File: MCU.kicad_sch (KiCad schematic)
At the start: 12 parts, among them IC2 PIC16F15345-I/SO, J5 490107670612

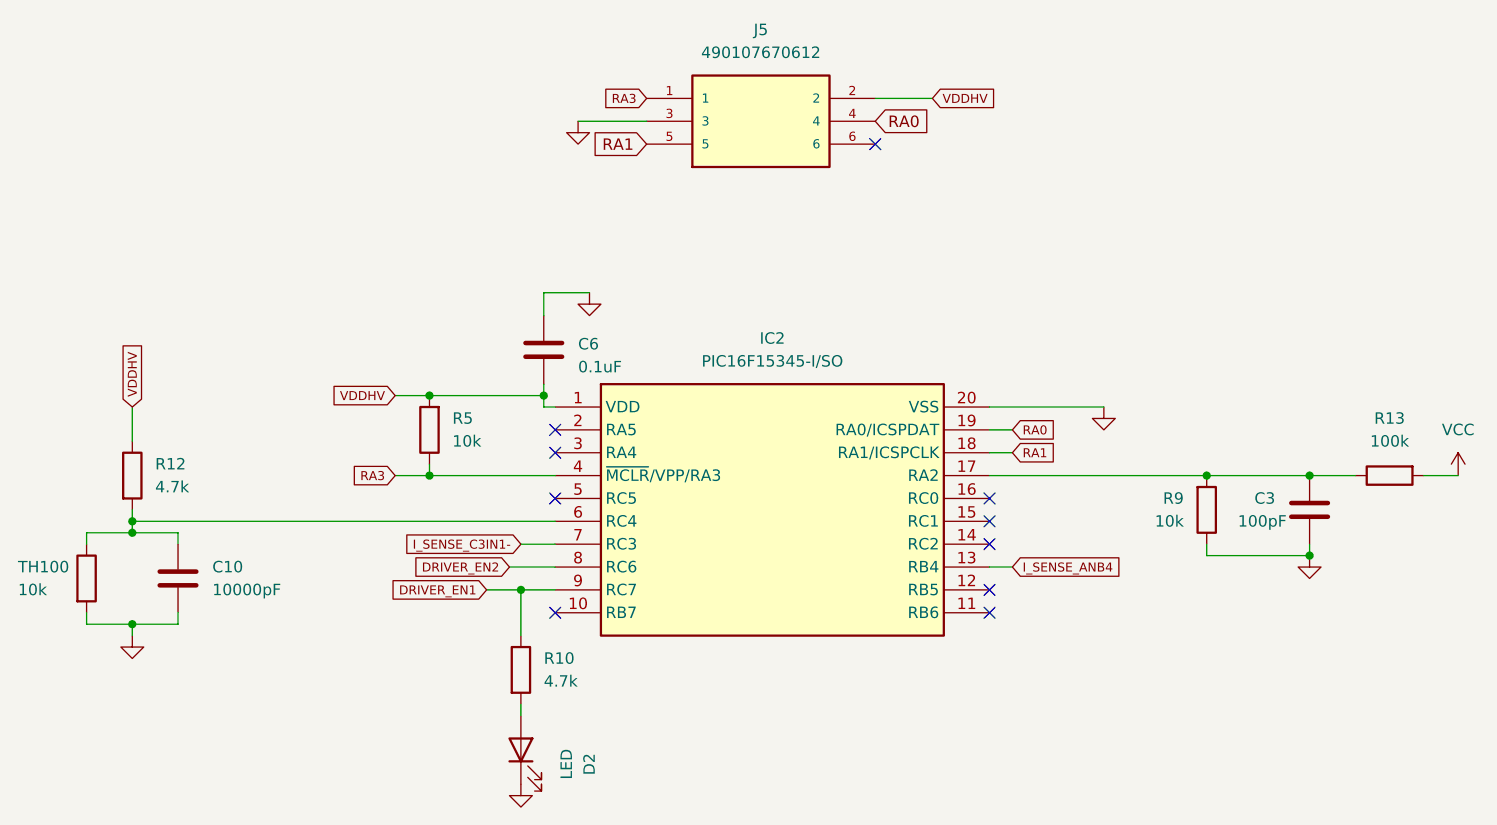
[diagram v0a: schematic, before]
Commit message: Final Design
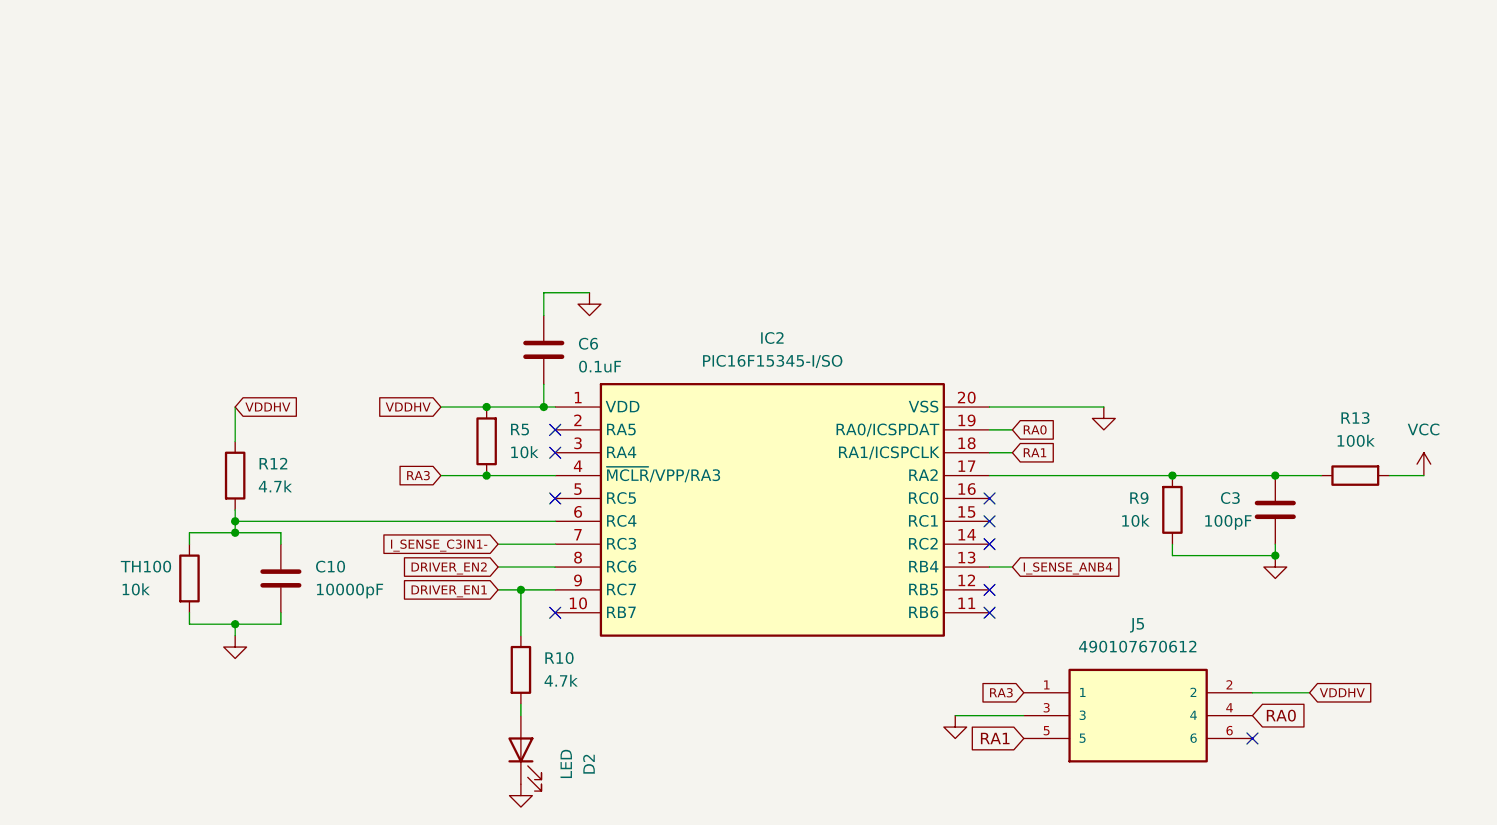
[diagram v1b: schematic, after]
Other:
- moved on the sheet: C10, C3, J5, R12, R13, R5, R9, TH100
